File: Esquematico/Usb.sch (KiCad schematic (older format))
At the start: 1 part

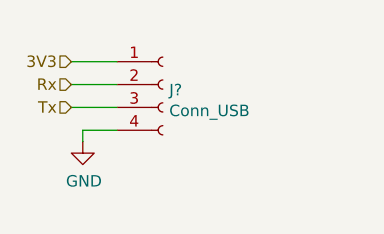
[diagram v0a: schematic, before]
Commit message: Foot prints
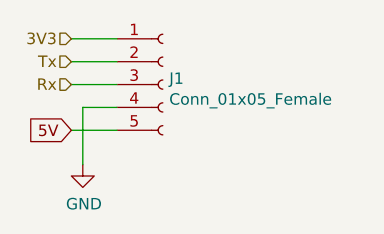
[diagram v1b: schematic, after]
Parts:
- removed J?: Conn_USB, symbol Connector:Conn_01x04_Female
- added J1: Conn_01x05_Female, symbol Connector:Conn_01x05_Female
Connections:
- net 3V3: now also J1.1 (Pin_1)
- net GND: now also J1.4 (Pin_4)
- net Rx: now also J1.3 (Pin_3)
- net Tx: now also J1.2 (Pin_2)
- new net 5V: J1.5 (Pin_5)
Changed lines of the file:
@@
 $EndDescr
 $Comp
-L power:GND #PWR?
+L power:GND #PWR0101
 U 1 1 61A9BEBF
-P 5950 3700
-F 0 "#PWR?" H 5950 3450 50  0001 C CNN
-F 1 "GND" H 5955 3527 50  0000 C CNN
-F 2 "" H 5950 3700 50  0001 C CNN
-F 3 "" H 5950 3700 50  0001 C CNN
-	1    5950 3700
+P 5950 3800
+F 0 "#PWR0101" H 5950 3550 50  0001 C CNN
+F 1 "GND" H 5955 3627 50  0000 C CNN
+F 2 "" H 5950 3800 50  0001 C CNN
+F 3 "" H 5950 3800 50  0001 C CNN
+	1    5950 3800
 	1    0    0    -1
 $EndComp
 Wire Wire Line
-	6100 3650 5950 3650
+	6100 3550 5950 3550
 Wire Wire Line
-	5950 3650 5950 3700
-Text HLabel 5900 3550 0    50   Input ~ 0
+	5950 3550 5950 3800
+Text HLabel 5900 3350 0    50   Input ~ 0
 Tx
 Text HLabel 5900 3450 0    50   Input ~ 0
@@
 	5900 3450 6100 3450
 Wire Wire Line
-	5900 3550 6100 3550
+	5900 3350 6100 3350
+Text HLabel 5900 3250 0    50   Input ~ 0
+3V3
+Wire Wire Line
+	5900 3250 6100 3250
 $Comp
-L Connector:Conn_01x04_Female J?
-U 1 1 61B53722
+L Connector:Conn_01x05_Female J1
+U 1 1 61B942FE
 P 6300 3450
-F 0 "J?" H 6328 3426 50  0000 L CNN
-F 1 "Conn_USB" H 6328 3335 50  0000 L CNN
+F 0 "J1" H 6328 3476 50  0000 L CNN
+F 1 "Conn_01x05_Female" H 6328 3385 50  0000 L CNN
 F 2 "" H 6300 3450 50  0001 C CNN
 F 3 "~" H 6300 3450 50  0001 C CNN
@@
 	1    0    0    -1
 $EndComp
-Text HLabel 5900 3350 0    50   Input ~ 0
-3V3
+Text GLabel 5900 3650 0    50   Input ~ 0
+5V
 Wire Wire Line
-	5900 3350 6100 3350
+	6100 3650 5900 3650
 $EndSCHEMATC
